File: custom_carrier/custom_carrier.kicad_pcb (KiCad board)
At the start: 2 copper layers, 2 parts, among them J1 ERF5-040-05.0-X-DV, J2 ERF5-040-05.0-X-DV

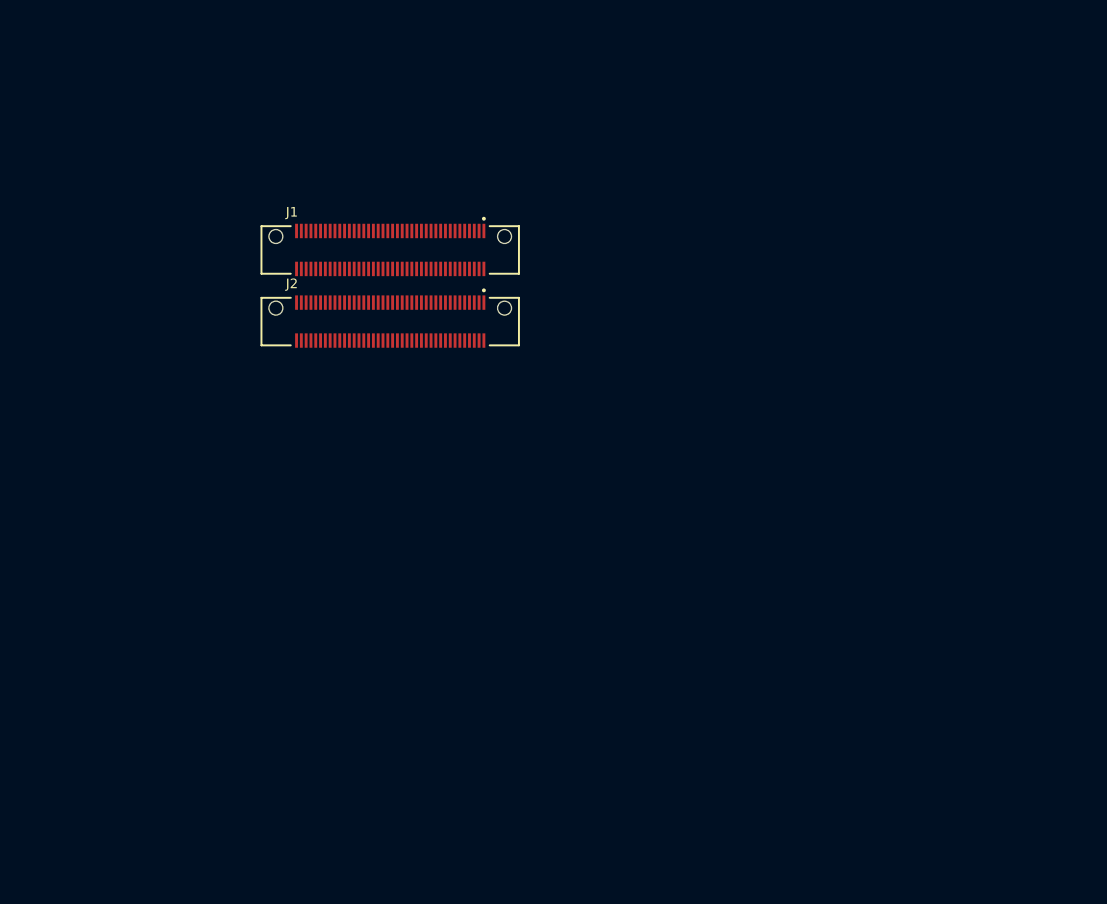
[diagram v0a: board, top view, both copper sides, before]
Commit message: working on custom carrier in V7
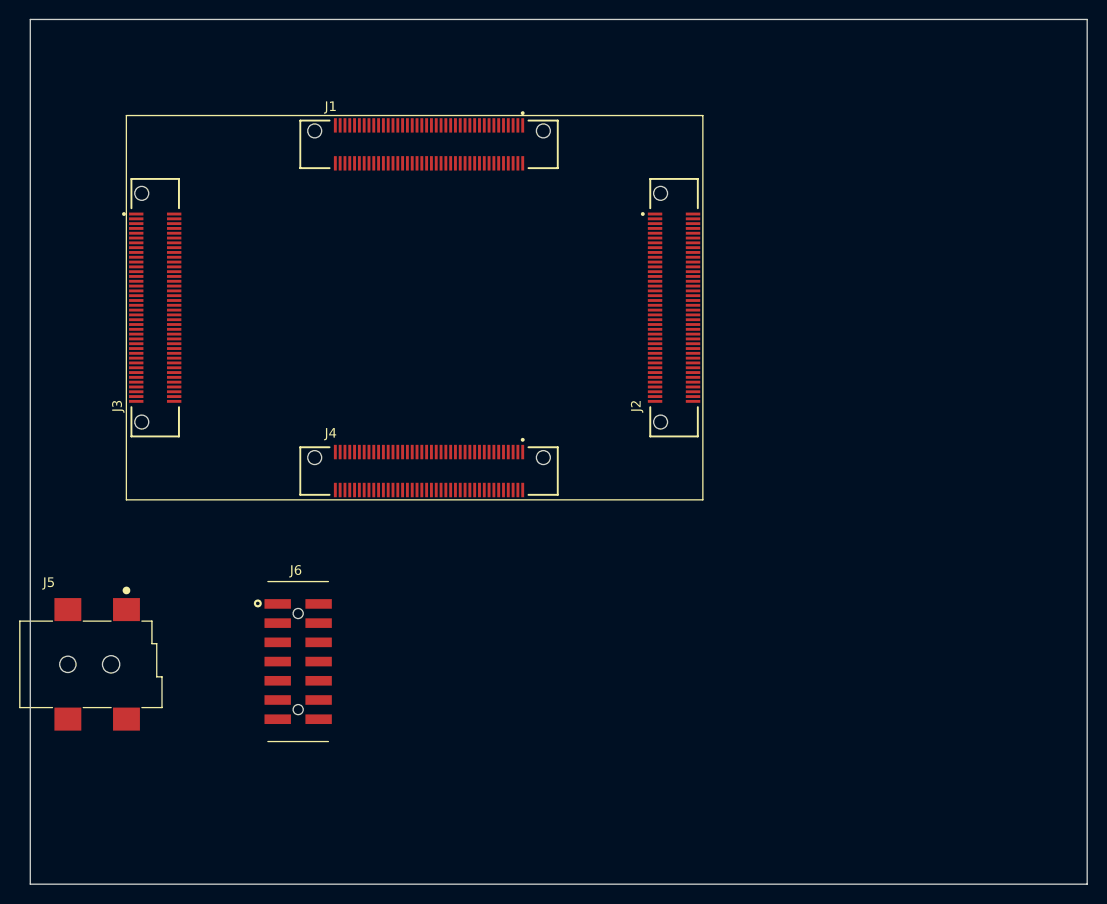
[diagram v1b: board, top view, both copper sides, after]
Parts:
- added J3: ERF5-040-05.0-X-DV, pedrolib:SAMTEC_ERF5-040-05.0-X-DV, F.Cu at (103.0, 100.0)
- added J4: ERF5-040-05.0-X-DV, pedrolib:SAMTEC_ERF5-040-05.0-X-DV, F.Cu at (131.5, 117.0)
- added J5: PJ-002AH-SMT-TR, pedrolib:CUI_PJ-002AH-SMT-TR, F.Cu at (100.0, 131.4)
- added J6: 87832-1420, pedrolib:MOLEX_87832-1420, F.Cu at (117.9, 136.8)
- moved J2 29.6 mm to (157.0, 100.0), turned to 90 degrees
- moved J1 11.7 mm to (131.5, 83.0)
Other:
- board outline added: 110 x 90 mm
